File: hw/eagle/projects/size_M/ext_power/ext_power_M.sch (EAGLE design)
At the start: 18 parts, among them T1 FDV304P

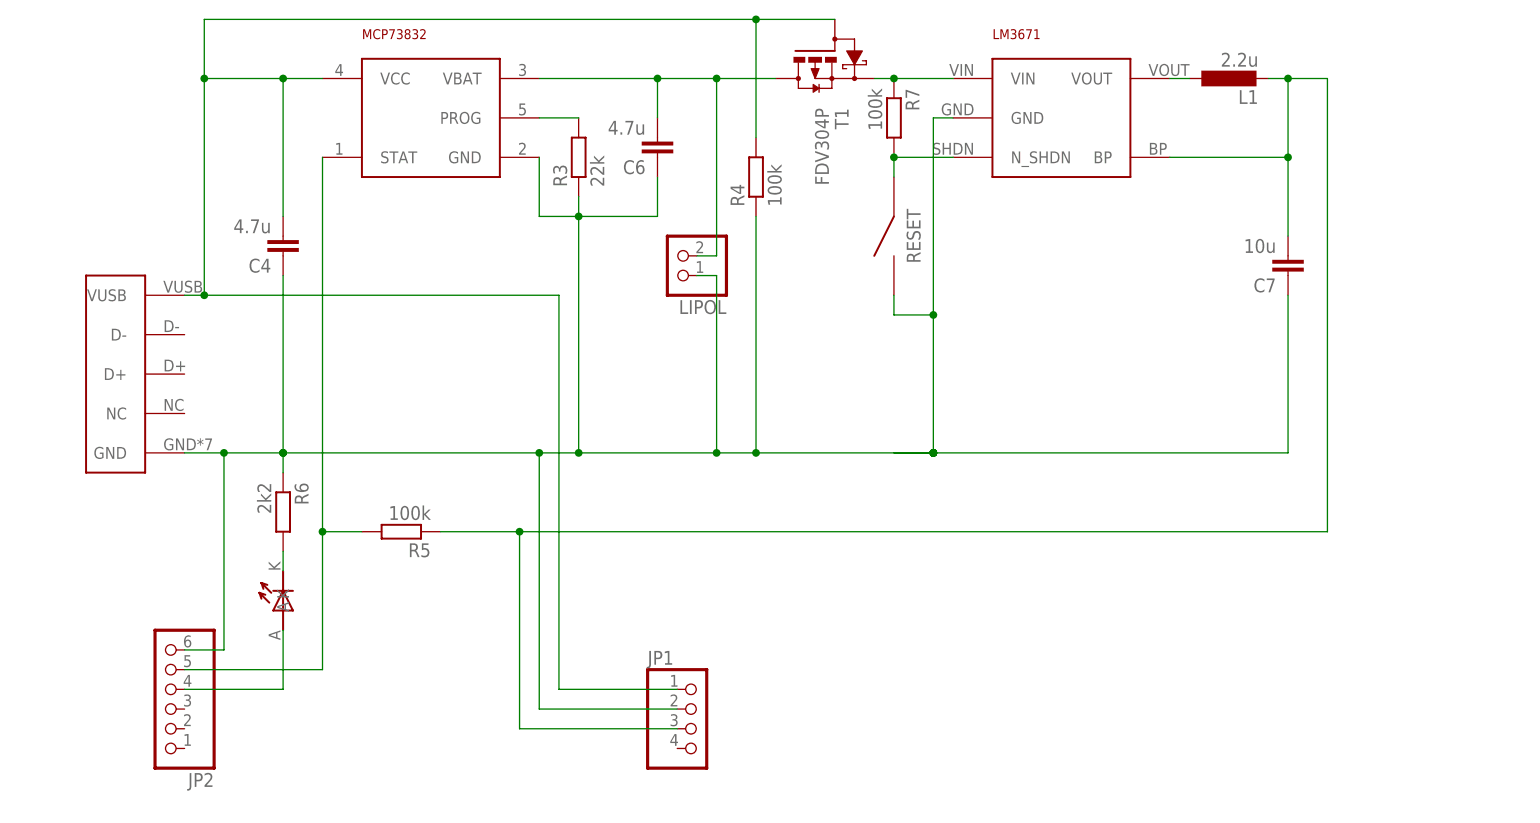
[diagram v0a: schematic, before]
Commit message: completed pcb design for M.0 - made PCB order
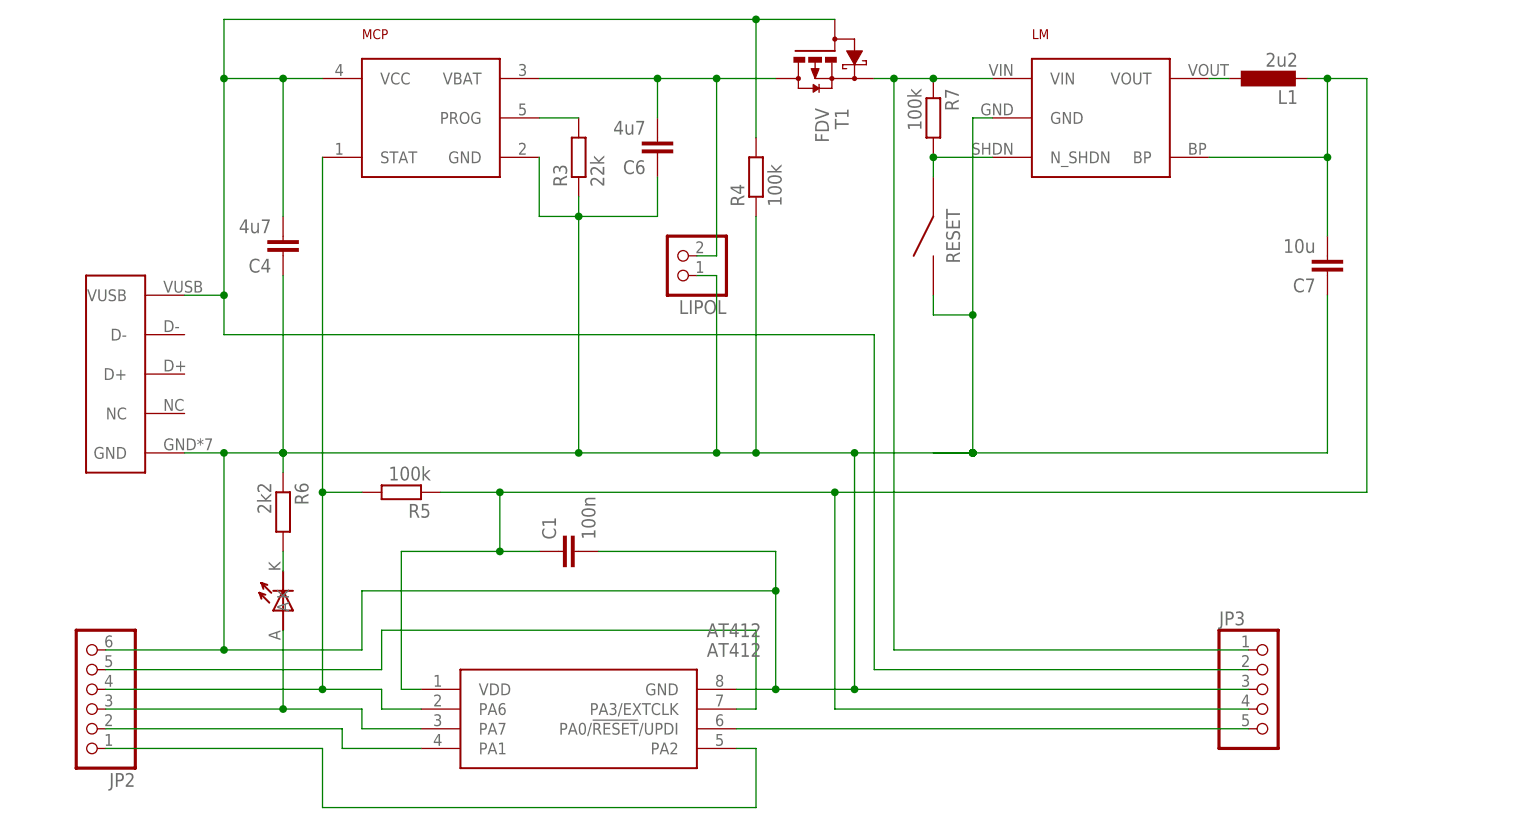
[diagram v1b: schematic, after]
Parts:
- removed JP1: (no value), pinhead2:PINHD-1X4
- removed LM3671: TC1185, !stavebnice03:STABILISER_APE8865
- added AT412: AT412, ATTINY412-SSN:ATTINY412-SSN
- added C1: 100n, rcl:C-EUC0603
- added JP3: (no value), pinhead2:PINHD-1X5
- added LM: TC, !stavebnice03:STABILISER_APE8865
- C4, C6: value 4.7u -> 4u7
- L1: value 2.2u -> 2u2
- MCP: value MCP73831 -> MCP
- T1: value FDV304P -> FDV
- renumbered MCP73832 to MCP
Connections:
- removed net N$1: D1.A, JP2.4
- removed net N$13: JP2.5, MCP.STAT, R5.2
- new net PA3: AT412.PA3/EXTCLK, JP2.5
- new net PA6: AT412.PA6, JP2.4, MCP.STAT, R5.2
- new net PA7: AT412.PA7, D1.A, JP2.3
- new net SCL: AT412.PA2, JP2.1
- new net SDA: AT412.PA1, JP2.2
- new net UPDI: AT412.PA0/!RESET!/UPDI, JP3.5
- net GND: now also AT412.GND, C1.2, JP3.3, LM.GND; no longer JP1.2, LM3671.GND
- net N$12: now also JP3.1, LM.VIN; no longer LM3671.VIN
- net N$2: now also LM.VOUT; no longer LM3671.VOUT
- net N$20: now also LM.N_SHDN; no longer LM3671.N_SHDN
- net N$9: now also JP3.2; no longer JP1.1
- net VDD: now also AT412.VDD, C1.1, JP3.4, LM.BP; no longer JP1.3, LM3671.BP
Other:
- moved on the sheet: C7, JP2, L1, R5, R7, RESET

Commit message: changes in pcb desingm - not finished and another minor changes in the documentation
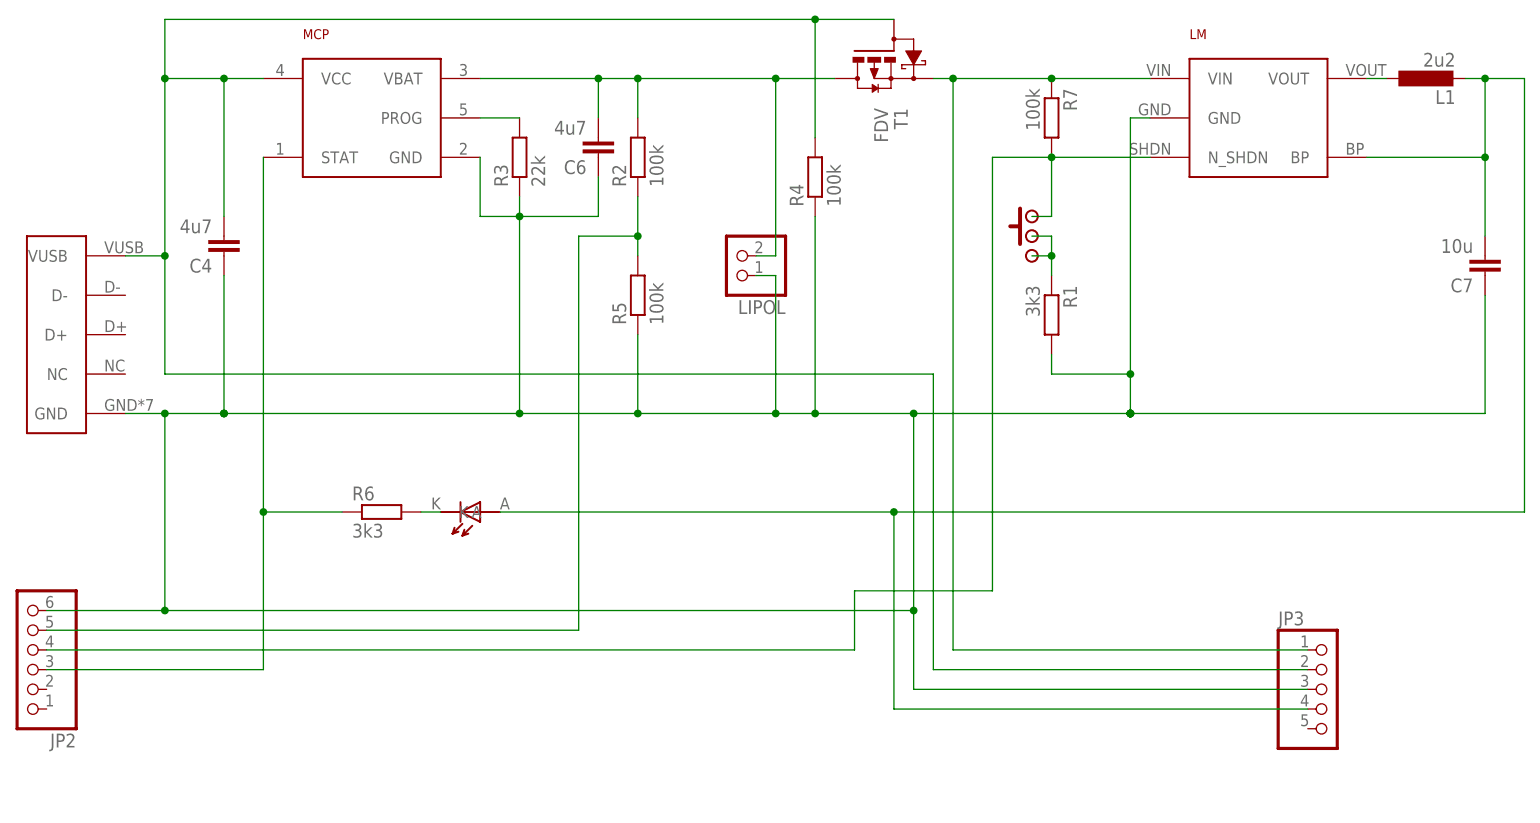
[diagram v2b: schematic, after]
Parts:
- removed AT412: AT412, ATTINY412-SSN:ATTINY412-SSN
- removed C1: 100n, rcl:C-EUC0603
- removed RESET: BYTTON-B3U, !stavebnice03:BYTTON-B3U
- added ON/OFF/RESET: SWITCH, hugo:SWITCH
- added R1: 3k3, rcl:R-EU_R0603
- added R2: 100k, rcl:R-EU_R0603
- R6: value 2k2 -> 3k3
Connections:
- removed net PA3: AT412.PA3/EXTCLK, JP2.5
- removed net PA6: AT412.PA6, JP2.4, MCP.STAT, R5.2
- removed net SCL: AT412.PA2, JP2.1
- removed net SDA: AT412.PA1, JP2.2
- removed net UPDI: AT412.PA0/!RESET!/UPDI, JP3.5
- new net N$1: ON/OFF/RESET.P$2, ON/OFF/RESET.P$3, R1.1
- new net N$5: JP2.5, R2.1, R5.2
- net GND: now also R1.2, R5.1; no longer AT412.GND, C1.2, R6.1, RESET.P$2
- net N$20: now also JP2.4, ON/OFF/RESET.P$1; no longer RESET.P$1
- net N$8: now also R2.2
- net PA7: now also MCP.STAT, R6.1; no longer AT412.PA7, D1.A
- net VDD: now also D1.A; no longer AT412.VDD, C1.1, R5.1
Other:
- moved on the sheet: C4, C6, C7, JP2, JP3, L1, LIPOL, LM, MCP, R3, R4, R5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
